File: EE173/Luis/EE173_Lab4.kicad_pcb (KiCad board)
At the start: 2 copper layers, 82.5 x 69.8 mm, 24 parts, among them J1 Conn_01x02_Male, J2 Conn_01x02_Male, J3 Test Line, J4 OSC, U1 74HC00, U2 L7806

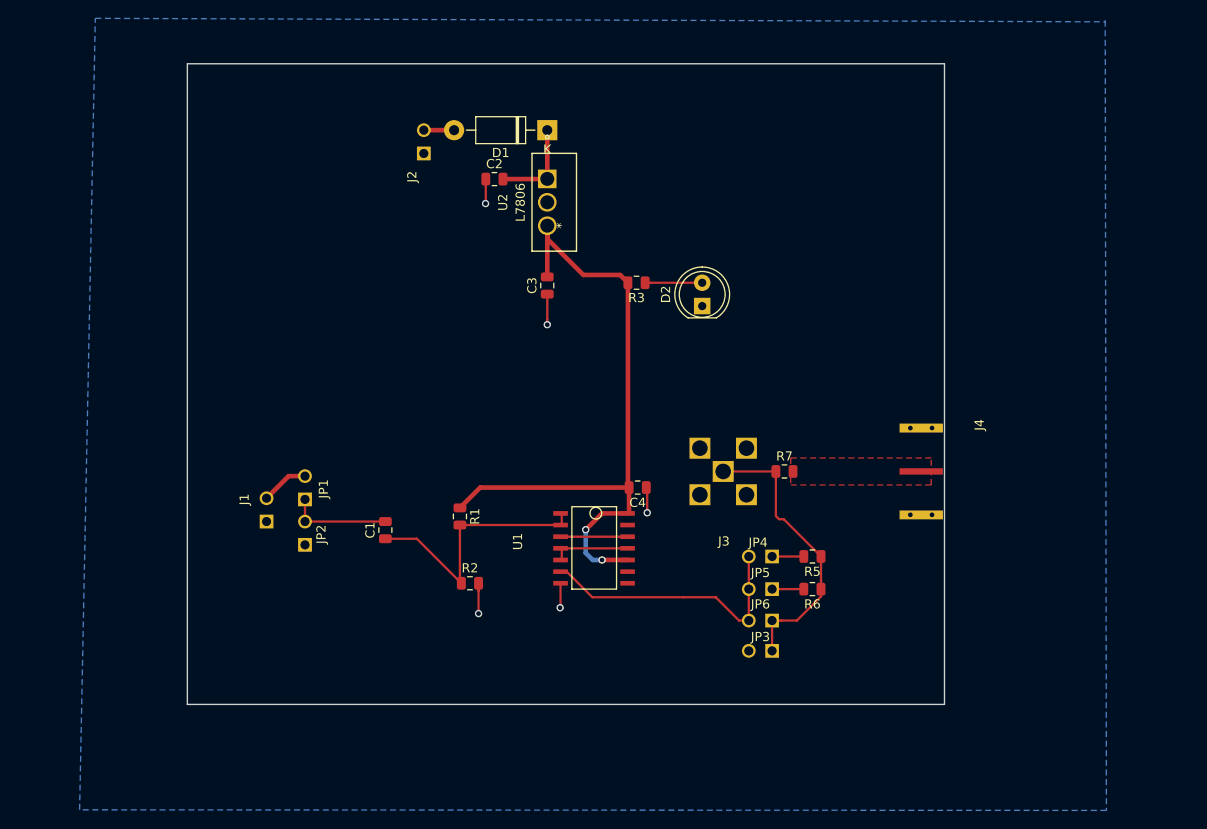
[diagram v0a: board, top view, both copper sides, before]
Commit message: added new HC00 Footprint under digikey.pretty
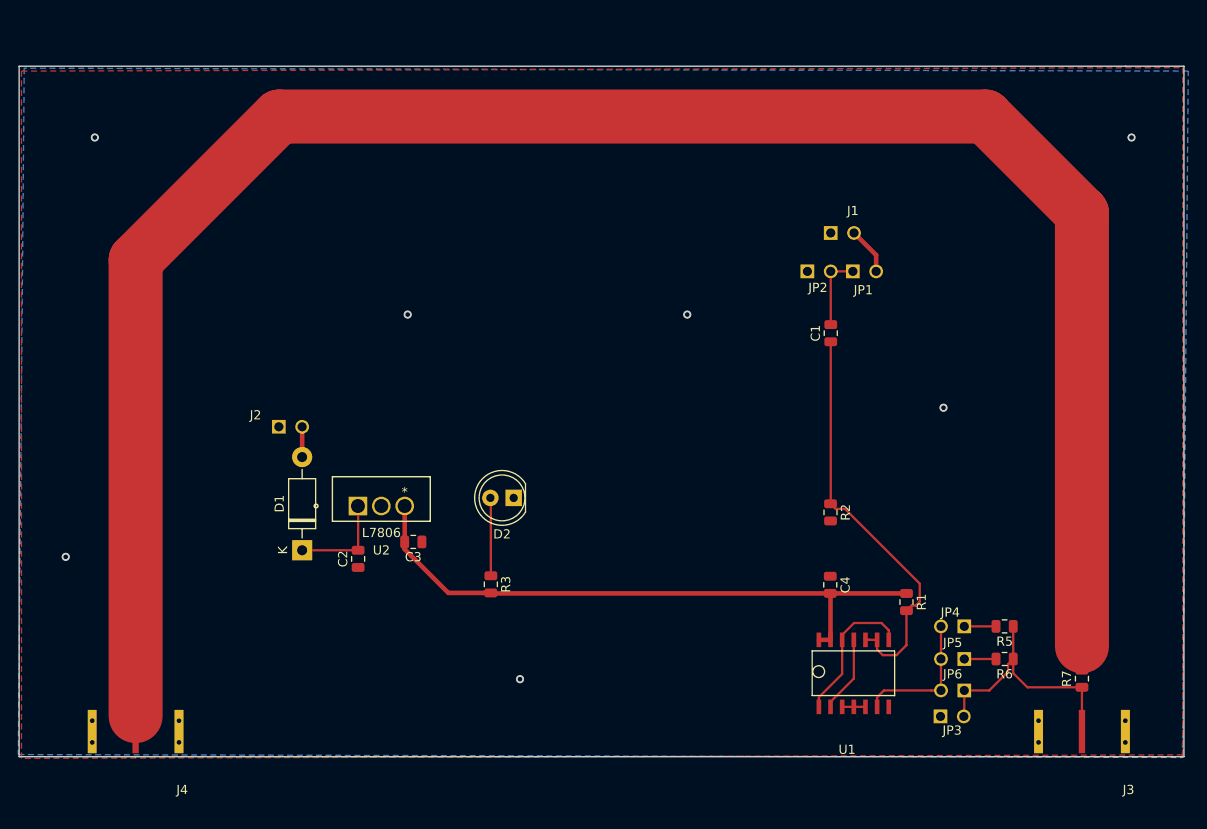
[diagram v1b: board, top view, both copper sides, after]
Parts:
- J3: footprint My_Footprints:Vertical_BNC_Connector -> My_Footprints:BNC_Connector
- moved J4 90.2 mm to (118.8, 112.2), turned to 0 degrees
- moved J1 70.3 mm to (197.1, 57.8), turned to 180 degrees
- moved JP1 66.2 mm to (199.6, 62.0), turned to 180 degrees
- moved JP2 63.5 mm to (194.6, 62.0), turned to 180 degrees
- moved C1 53.1 mm to (194.6, 68.7)
- moved D1 53.0 mm to (137.0, 92.4), turned to 90 degrees
- moved R1 49.6 mm to (202.9, 98.1)
- moved J3 48.3 mm to (222.0, 112.2)
- moved C2 44.0 mm to (143.1, 93.4), turned to 90 degrees
- moved R2 40.1 mm to (194.6, 88.3), turned to 270 degrees
- moved R7 39.5 mm to (222.0, 106.4), turned to 90 degrees
- moved R3 36.5 mm to (157.6, 96.1), turned to 270 degrees
- moved U1 35.2 mm to (194.6, 109.3), turned to 0 degrees
- moved J2 35.0 mm to (137.0, 78.9), turned to 180 degrees
- moved U2 33.7 mm to (148.2, 86.1), turned to 0 degrees
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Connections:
- JP3 pad 1: GND -> Net-(J3-Pad1)
- JP3 pad 2: Net-(J3-Pad1) -> GND
- U1 pad 1: Net-(C1-Pad1) -> Net-(U1-Pad1)
- U1 pad 10: +6V -> Net-(C1-Pad1)
- U1 pad 12: Net-(U1-Pad12) -> Net-(U1-Pad1)
- U1 pad 13: Net-(U1-Pad13) -> +6V
- U1 pad 2: Net-(C1-Pad1) -> Net-(U1-Pad11)
- U1 pad 3: Net-(U1-Pad12) -> Net-(U1-Pad3)
- U1 pad 4: Net-(U1-Pad11) -> Net-(U1-Pad3)
- U1 pad 5: Net-(U1-Pad11) -> Net-(U1-Pad3)
- U1 pad 8: Net-(U1-Pad13) -> Net-(U1-Pad1)
- U1 pad 9: Net-(U1-Pad12) -> Net-(C1-Pad1)
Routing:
- net Net-(J4-Pad1): track 0.00 -> 211.0 mm
- net Net-(C1-Pad1): track 29.1 -> 45.3 mm
- net Net-(U1-Pad1): track 0.00 -> 15.9 mm
- net GND: track 14.5 -> 0.00 mm, vias 5 -> 7
- net Net-(JP4-Pad1): track 29.6 -> 15.3 mm
- net Net-(U1-Pad12): track 8.39 -> 0.00 mm
- net +6V: track 75.5 -> 67.9 mm, vias 2 -> 0
- net Net-(J3-Pad1): track 31.4 -> 28.2 mm
- net Net-(C1-Pad2): track 11.2 -> 8.21 mm
- net Net-(U1-Pad3): track 0.00 -> 2.54 mm
- net Net-(D2-Pad2): track 6.22 -> 8.51 mm
- net Net-(C2-Pad2): track 10.1 -> 10.9 mm
- net Net-(U1-Pad13): track 0.54 -> 0.00 mm
- added copper zone on F.Cu, net GND
- removed copper zone on F.Cu, net Net-(J4-Pad1)
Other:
- board size 82.5 x 69.8 mm -> 127 x 75.3 mm
- rule trace_min: 0.2 -> 1.27
- rule via_min_size: 0.4 -> 0.508
